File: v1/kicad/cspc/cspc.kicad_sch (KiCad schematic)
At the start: 16 parts, among them J1 LNCPU_FLAGS_Connector, U1 LNCPU Type A Connector, U10 74LS169, U11 74LS169, U12 74LS169, U13 74LS169, U14 74LS32, U15 74LS04, U2 74LS155, U3 74LS04, U4 74LS32, U5 74LS32, U6 74LS157, U7 74LS157, U8 74LS157, U9 74LS157

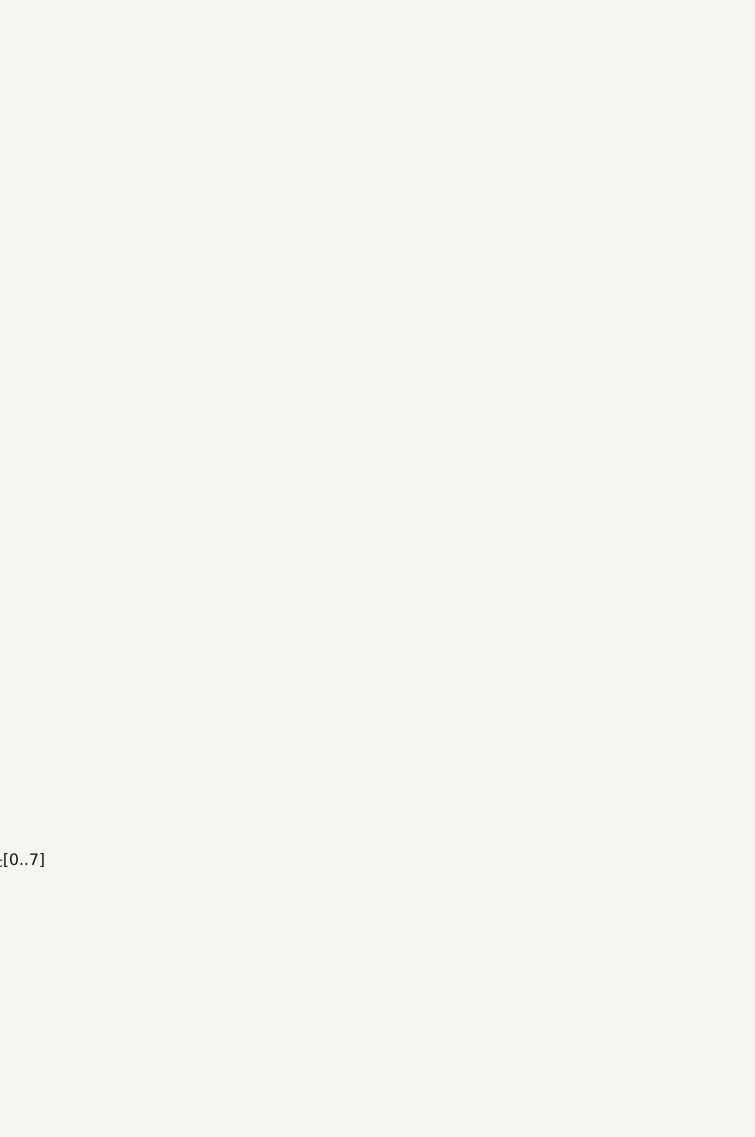
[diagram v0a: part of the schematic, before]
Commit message: PARTIAL
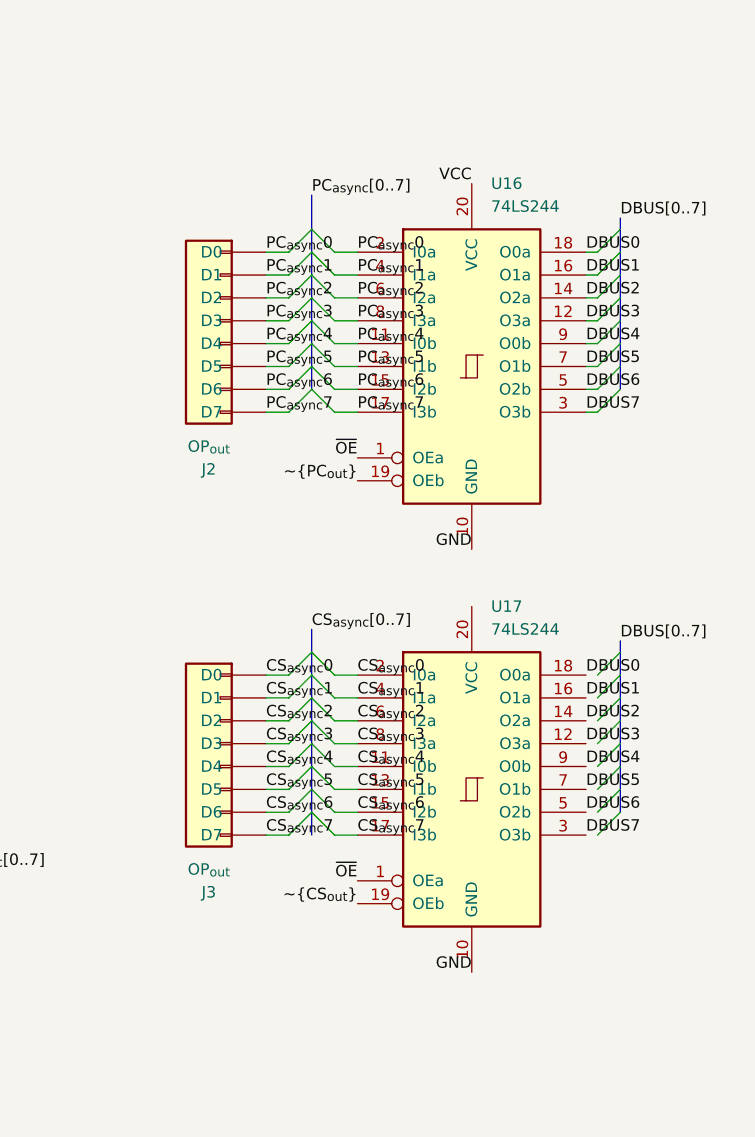
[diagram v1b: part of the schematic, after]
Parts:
- added J2, J3: OP_{out}, Connector_PinSocket_2.54mm:PinSocket_1x08_P2.54mm_Vertical, symbol lncpu:LNCPU_DBUS_Socket
- added U16, U17: 74LS244, Package_DIP:DIP-20_W7.62mm_LongPads, symbol 74xx:74LS244
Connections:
- net CS_{async}0: now also J3.1 (D0), U17.2 (I0a)
- net CS_{async}1: now also J3.2 (D1), U17.4 (I1a)
- net CS_{async}2: now also J3.3 (D2), U17.6 (I2a)
- net CS_{async}3: now also J3.4 (D3), U17.8 (I3a)
- net CS_{async}4: now also J3.5 (D4), U17.11 (I0b)
- net CS_{async}5: now also J3.6 (D5), U17.13 (I1b)
- net CS_{async}6: now also J3.7 (D6), U17.15 (I2b)
- net CS_{async}7: now also J3.8 (D7), U17.17 (I3b)
- net DBUS0: now also U16.18 (O0a), U17.18 (O0a)
- net DBUS1: now also U16.16 (O1a), U17.16 (O1a)
- net DBUS2: now also U16.14 (O2a), U17.14 (O2a)
- net DBUS3: now also U16.12 (O3a), U17.12 (O3a)
- net DBUS4: now also U16.9 (O0b), U17.9 (O0b)
- net DBUS5: now also U16.7 (O1b), U17.7 (O1b)
- net DBUS6: now also U16.5 (O2b), U17.5 (O2b)
- net DBUS7: now also U16.3 (O3b), U17.3 (O3b)
- net GND: now also U16.10 (GND), U17.10 (GND)
- net PC_{async}0: now also J2.1 (D0), U16.2 (I0a)
- net PC_{async}1: now also J2.2 (D1), U16.4 (I1a)
- net PC_{async}2: now also J2.3 (D2), U16.6 (I2a)
- net PC_{async}3: now also J2.4 (D3), U16.8 (I3a)
- net PC_{async}4: now also J2.5 (D4), U16.11 (I0b)
- net PC_{async}5: now also J2.6 (D5), U16.13 (I1b)
- net PC_{async}6: now also J2.7 (D6), U16.15 (I2b)
- net PC_{async}7: now also J2.8 (D7), U16.17 (I3b)
- net VCC: now also U16.20 (VCC)
- net ~{CS_{out}}: now also U17.19 (OEb)
- net ~{OE}: now also U16.1 (OEa), U17.1 (OEa)
- net ~{PC_{out}}: now also U16.19 (OEb)
